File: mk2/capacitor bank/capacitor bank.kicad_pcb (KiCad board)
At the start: 2 copper layers, 228.6 x 61 mm, 13 parts

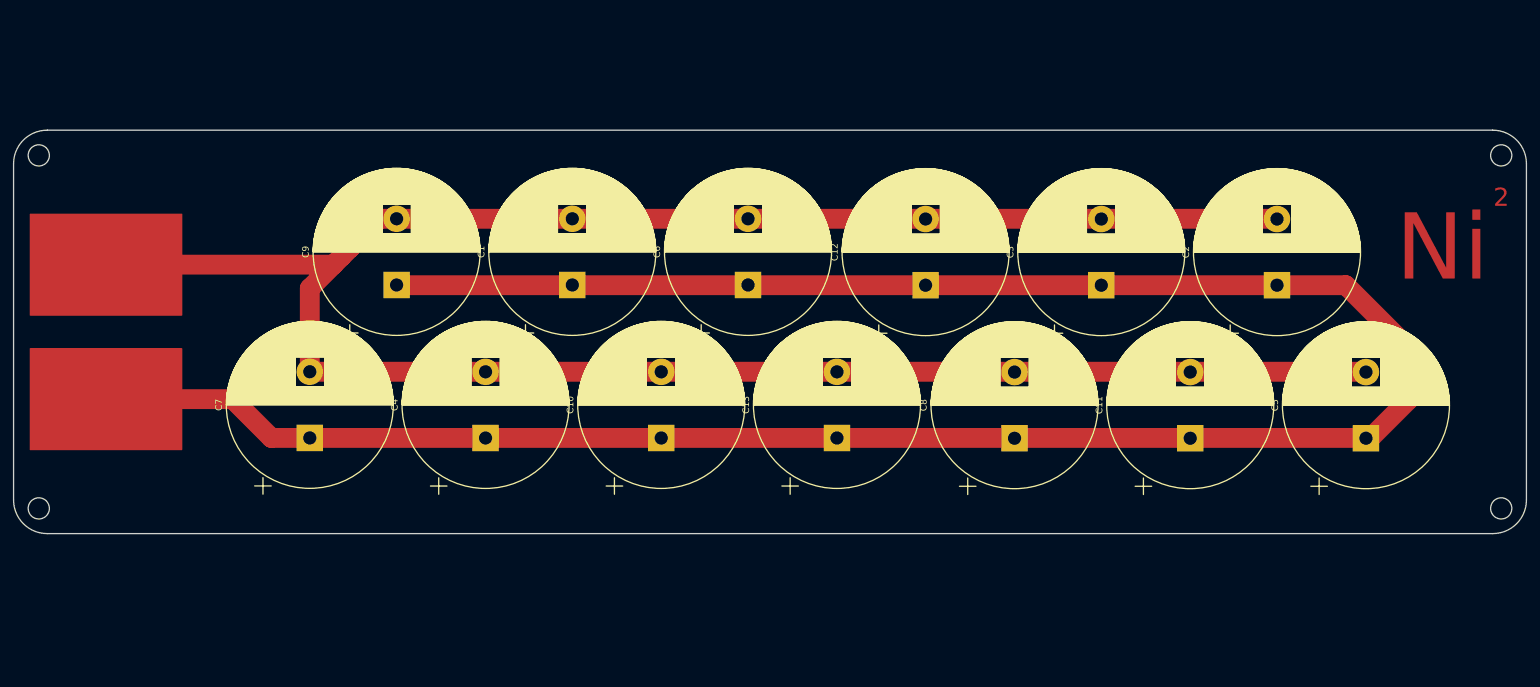
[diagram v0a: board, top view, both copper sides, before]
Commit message: Work updates
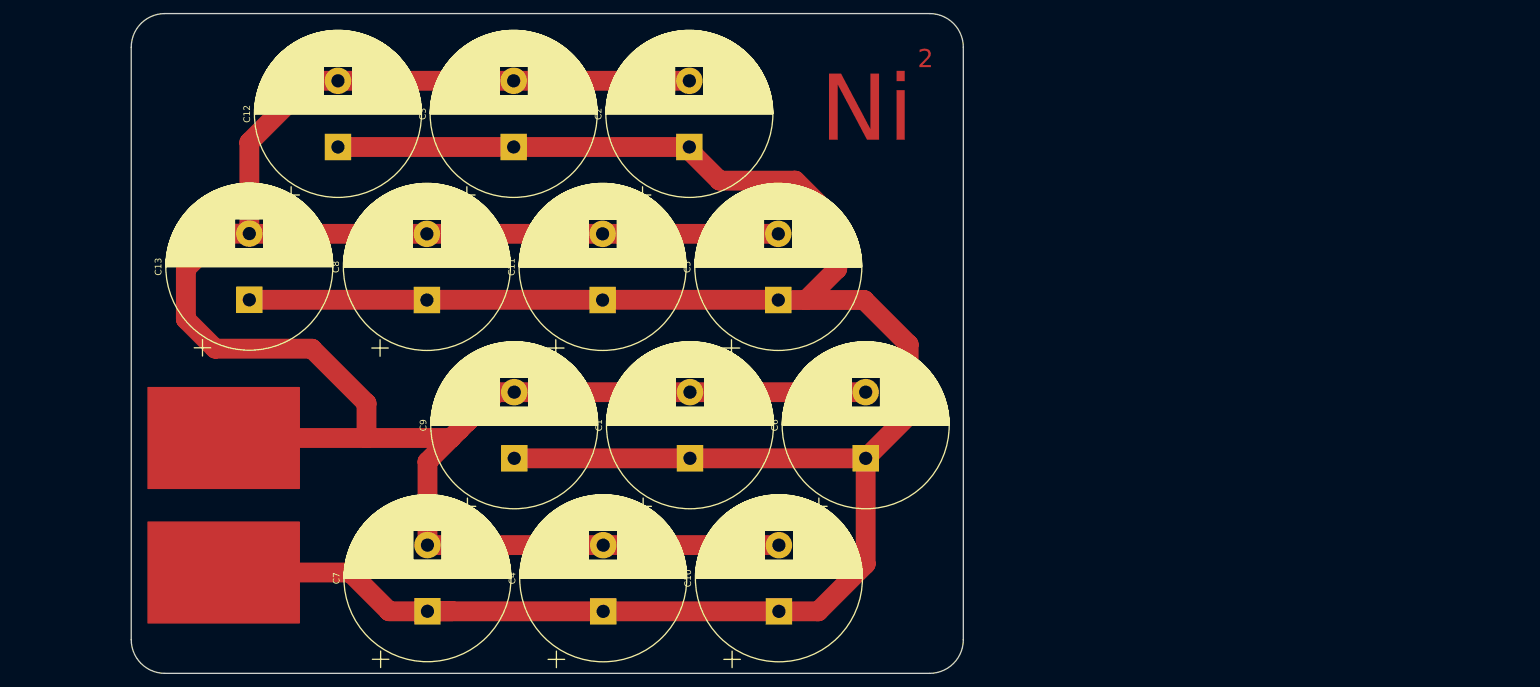
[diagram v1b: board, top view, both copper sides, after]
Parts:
- moved C2 91.2 mm to (142.8, 58.4)
- moved C5 91.2 mm to (156.2, 81.5)
- moved C3 91.2 mm to (116.2, 58.4)
- moved C11 91.2 mm to (129.6, 81.5)
- moved C12 91.2 mm to (89.7, 58.4)
- moved C13 91.2 mm to (76.3, 81.5)
- moved C8 91.2 mm to (103.1, 81.5)
- moved C1 31.7 mm to (142.8, 105.5)
- moved C10 31.7 mm to (156.3, 128.6)
- moved C4 31.7 mm to (129.7, 128.6)
- moved C6 31.7 mm to (169.4, 105.5)
- moved C9 31.7 mm to (116.3, 105.5)
- moved C7 31.7 mm to (103.2, 128.6)
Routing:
- net Net-(C1-Pad2): track 345.7 -> 380.6 mm
- net Net-(C1-Pad1): track 355.0 -> 380.4 mm
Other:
- board size 228.6 x 61 mm -> 125.7 x 99.7 mm
